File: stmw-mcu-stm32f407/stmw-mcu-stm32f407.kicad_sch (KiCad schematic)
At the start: 41 parts, among them J2 TYPE-C-31-M-12, SW1 TS-1088R-02526, SW2 TS-1088R-02526, U1 AMS1117-3.3, U3 STM32F407VETx, Y1 X_16MHZ

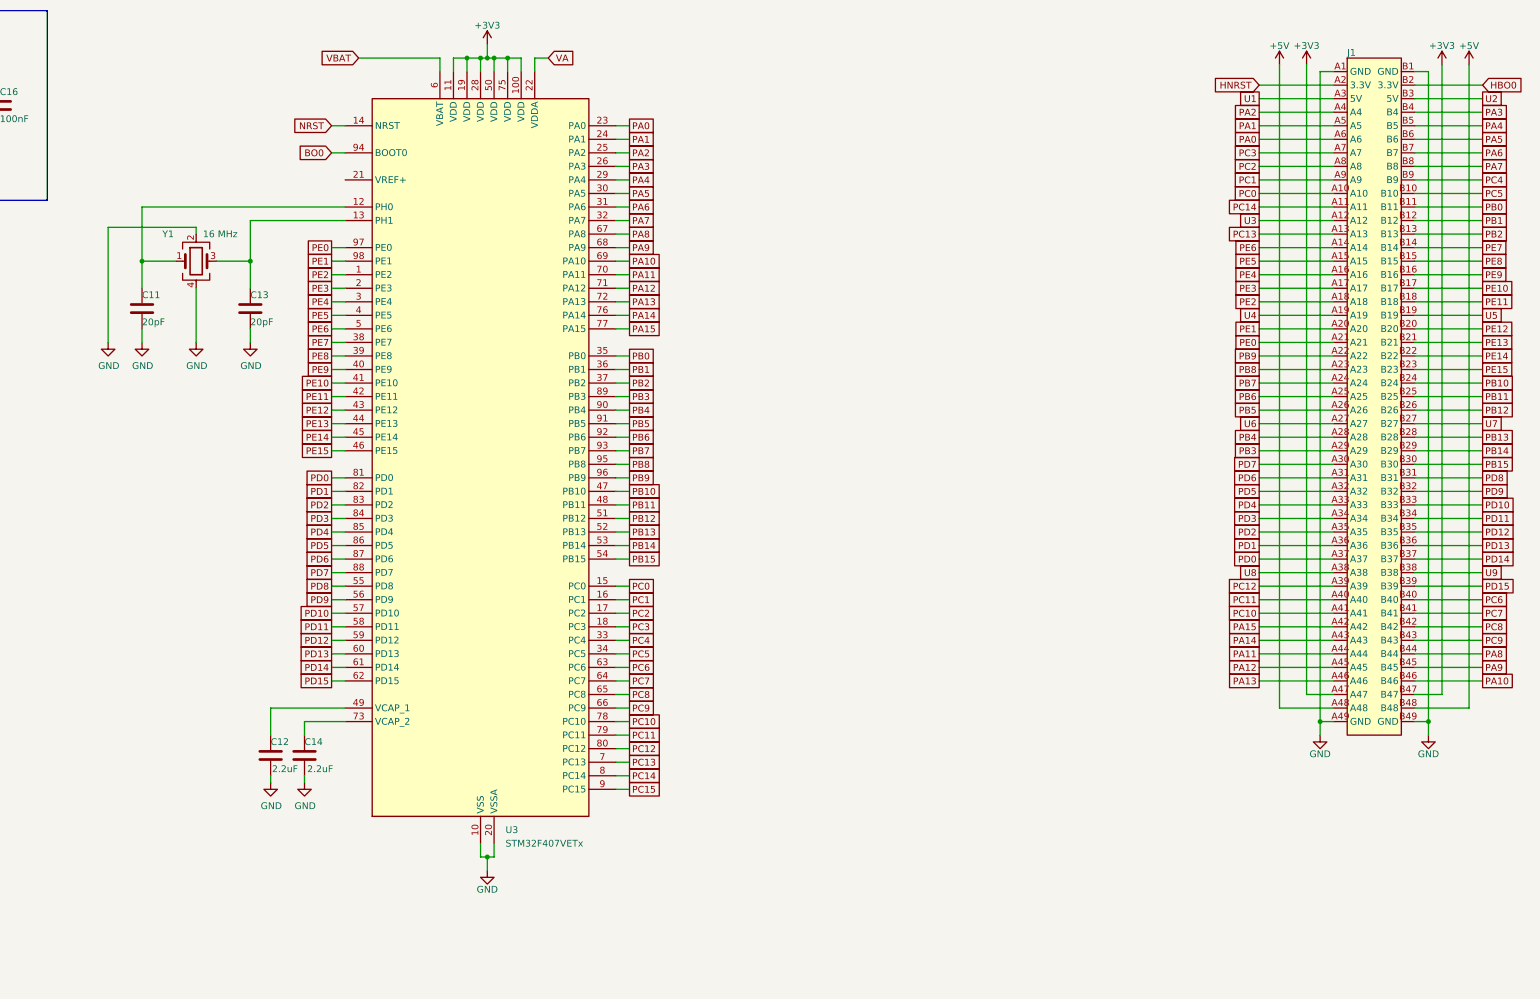
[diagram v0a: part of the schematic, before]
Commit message: Hmmm
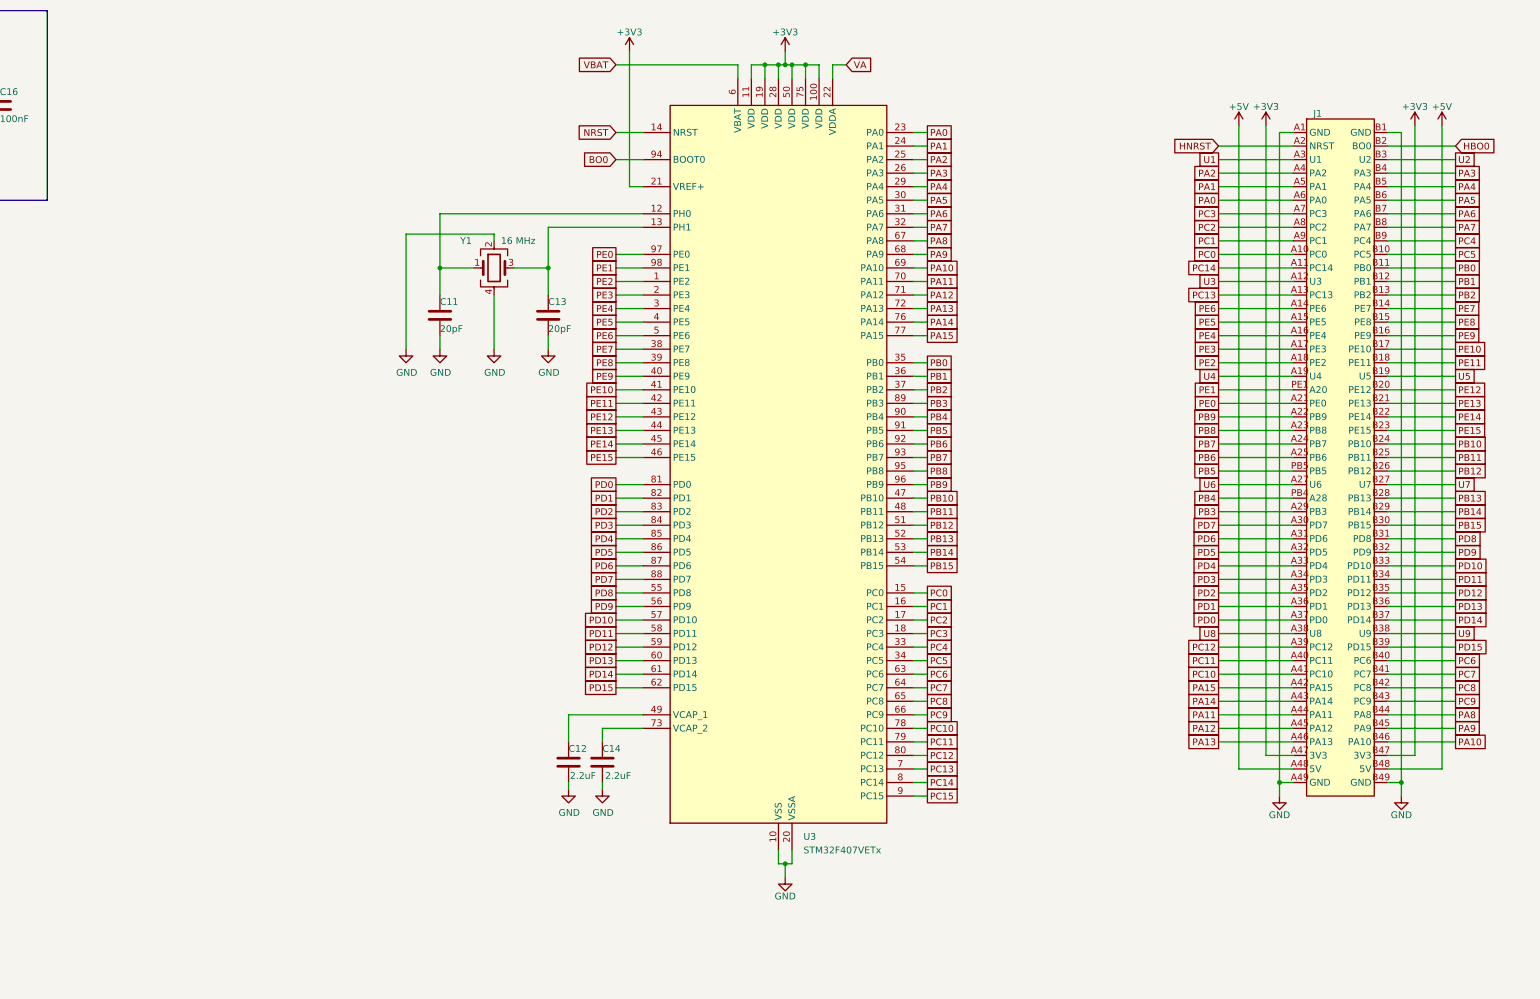
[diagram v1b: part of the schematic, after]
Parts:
- C1, C3: value C_10UF_0805 -> 10uF
- C10, C15, C16, C2, C5, C6, C7, C8, C9: value C_100NF_0603 -> 100nF
- C11, C13: value C_20PF_0603 -> 20pF
- C4: value C_1UF_0603 -> 1uF
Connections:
- net +3V3: now also U3.21 (VREF+)
- net PB4: now also J1.PB4 (A28); no longer J1.A28
- net PB5: now also J1.PB5; no longer J1.A26
- net PE1: now also J1.PE1 (A20); no longer J1.A20
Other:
- moved on the sheet: C11, C12, C13, C14, J1, U3, Y1
